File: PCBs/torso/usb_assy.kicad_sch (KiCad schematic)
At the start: 5 parts, among them J3 USB_B_Micro

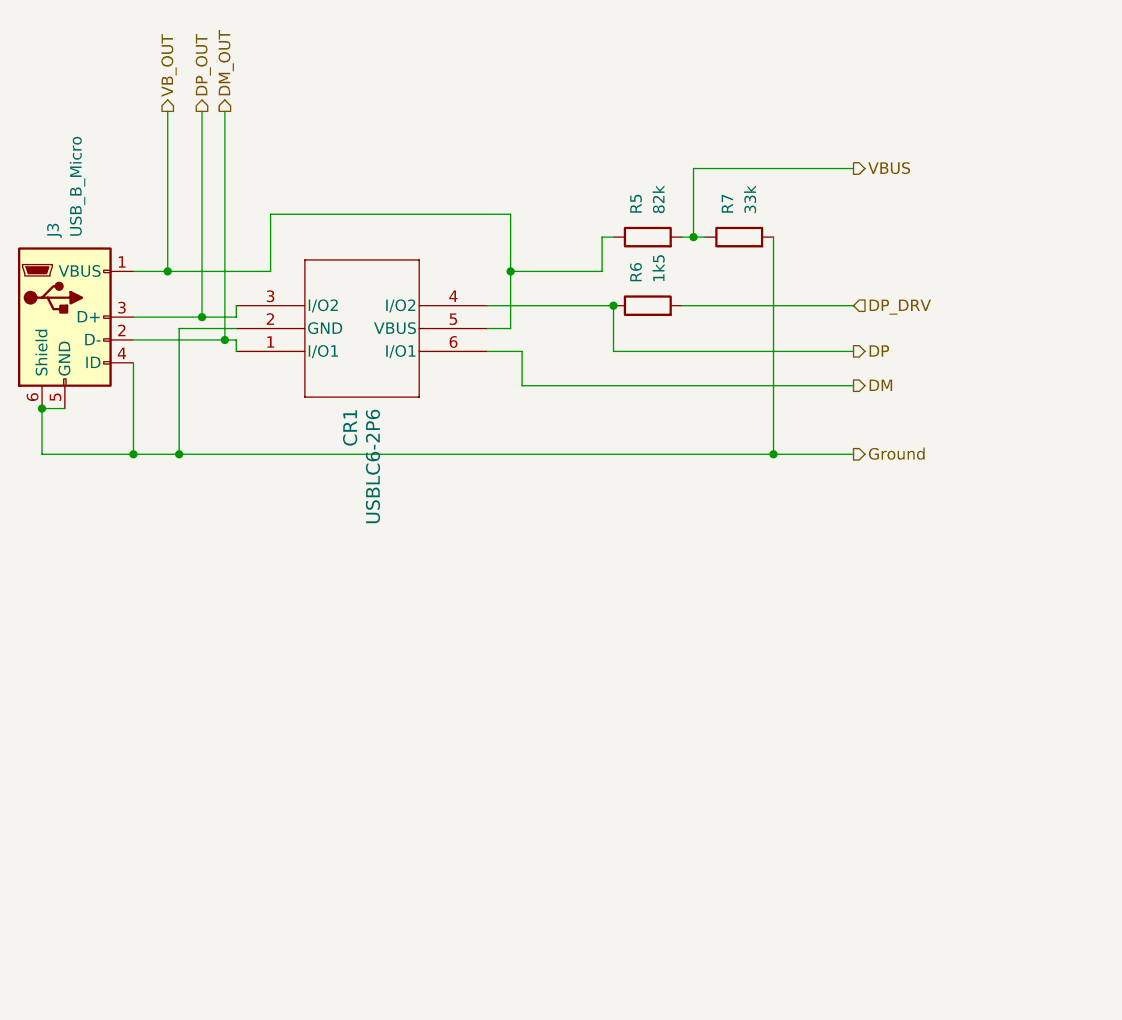
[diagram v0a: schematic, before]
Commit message: Added pcb pdfs
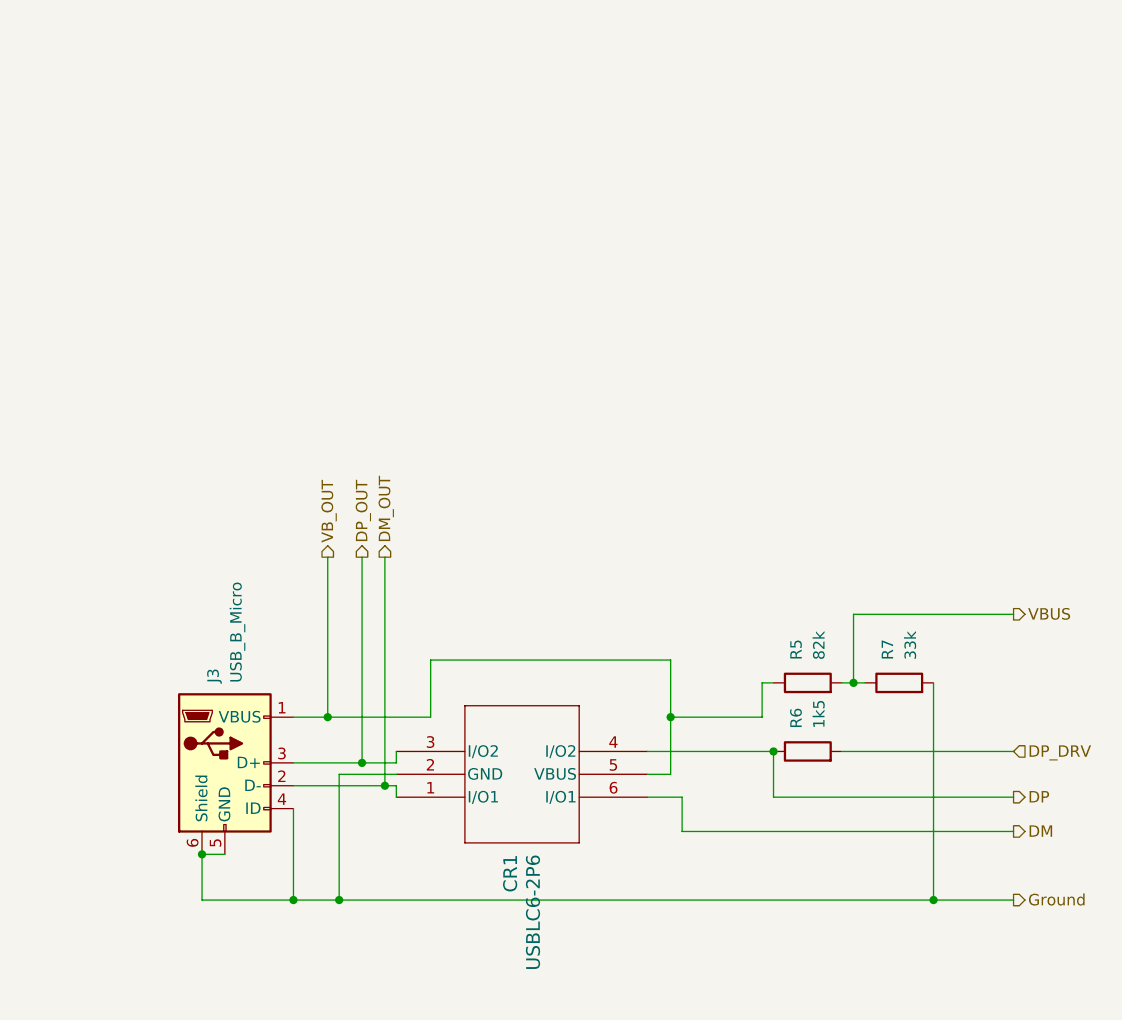
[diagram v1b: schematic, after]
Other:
- moved on the sheet: CR1, J3, R5, R6, R7
